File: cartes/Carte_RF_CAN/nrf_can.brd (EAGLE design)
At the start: 32.7 x 41.9 mm, 14 parts, among them Q1 16MHz

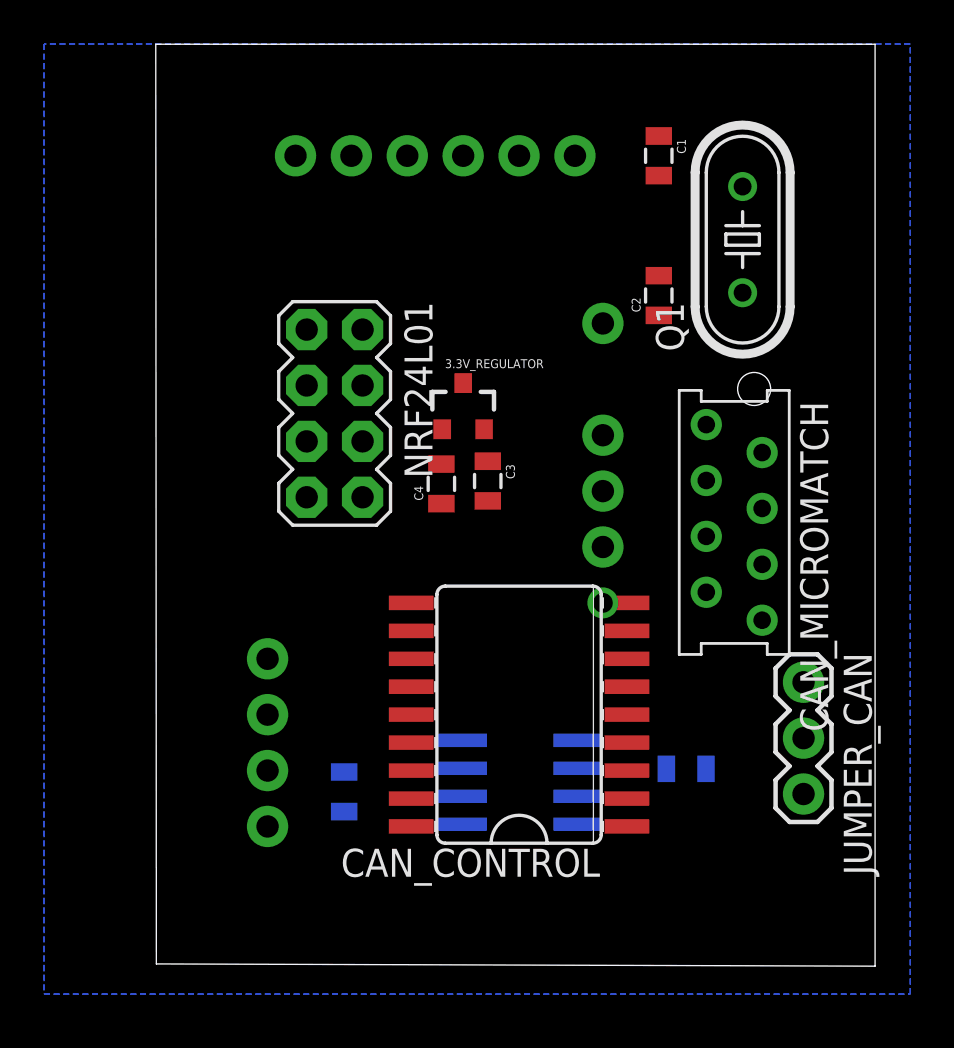
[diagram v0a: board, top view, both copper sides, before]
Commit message: finit rf
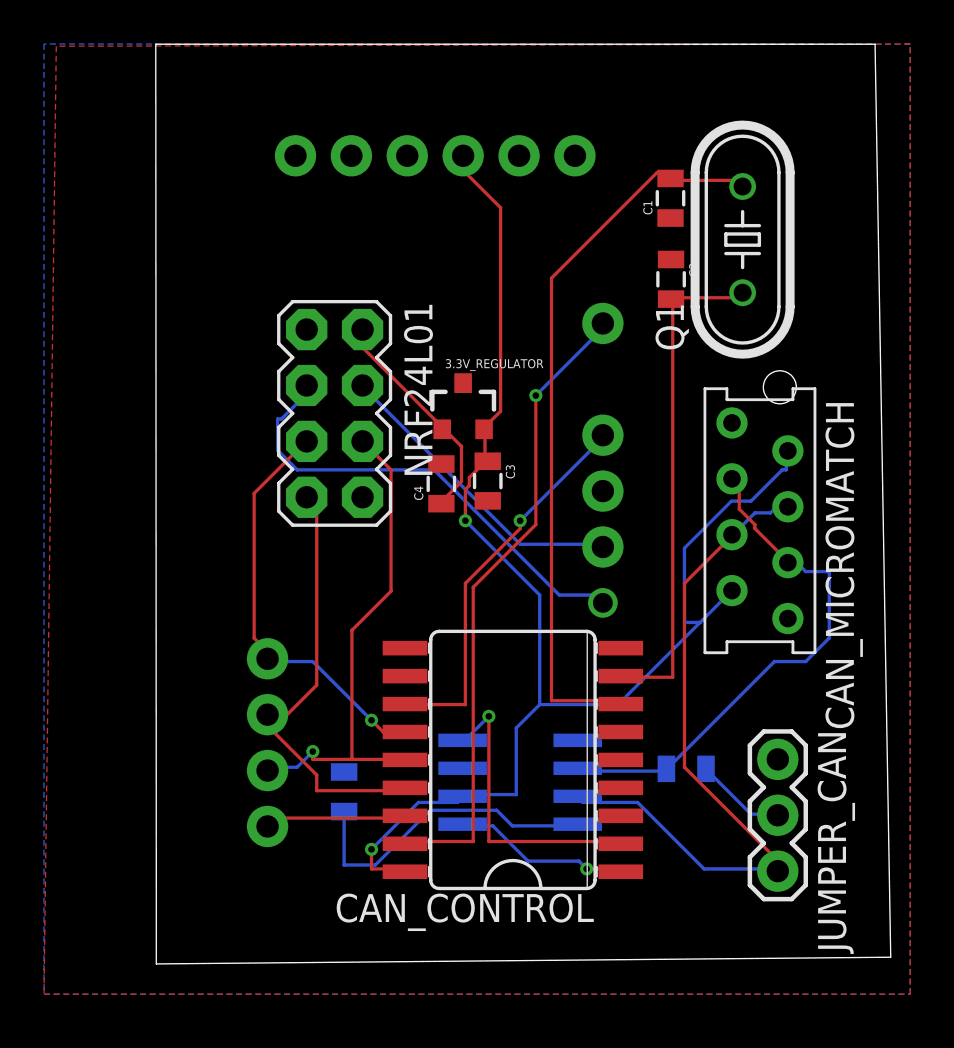
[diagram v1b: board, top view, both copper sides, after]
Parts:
- moved JUMPER_CAN 3.69 mm to (35.9, 19.6)
- moved CAN_CONTROL 2.08 mm to (23.9, 19.5)
- moved C1 2.00 mm to (31.0, 45.1), turned to 90 degrees
- moved CAN_MICROMATCH 1.17 mm to (35.1, 34.8)
- moved C2 0.92 mm to (31.0, 41.4), turned to 270 degrees
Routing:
- net VCC: track 0.00 -> 64.5 mm, vias 0 -> 2
- net N$2: track 0.00 -> 33.6 mm
- net CANH: track 0.00 -> 31.5 mm
- net RST: track 0.00 -> 29.3 mm, vias 0 -> 1
- net CANL: track 0.00 -> 24.1 mm
- net N$3: track 0.00 -> 23.0 mm
- net MOSI: track 0.00 -> 22.7 mm, vias 0 -> 1
- net NRF_CE: track 0.00 -> 21.2 mm
- net MISO: track 0.00 -> 21.0 mm
- net SCK: track 0.00 -> 18.8 mm, vias 0 -> 1
- net CAN_INT: track 0.00 -> 17.6 mm, vias 0 -> 1
- net N$5: track 0.00 -> 14.4 mm
- net NRF_CSN: track 0.00 -> 14.0 mm
- net CAN_RXD: track 0.00 -> 13.4 mm, vias 0 -> 1
- net 3.3V: track 0.00 -> 10.2 mm
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- added copper zone on layer 1, net GND
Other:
- board size 32.7 x 41.9 mm -> 33.4 x 41.8 mm
